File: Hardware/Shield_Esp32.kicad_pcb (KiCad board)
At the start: 2 copper layers, 93 x 70.5 mm, 43 parts, among them J1 Conn_01x02_Male, J10 Conn_01x02_Male, J11 Conn_01x02_Male, J12 Conn_01x02_Male, J13 Conn_01x02_Male, J14 Conn_01x02_Male, J15 Conn_01x02_Male, J16 Conn_01x02_Male, J17 Conn_01x02_Male, J18 Conn_01x02_Male, J19 Conn_01x02_Male, J2 Conn_01x02_Male, J20 Conn_01x02_Male, J21 Conn_01x02_Male, J22 Conn_01x02_Male, J23 Conn_01x02_Male, J3 Conn_02x13_Odd_Even, J4 Conn_01x15, J5 Conn_01x15, J6 Conn_01x02_Male, J7 Conn_01x02_Male, J8 Conn_01x03_Male, J9 Conn_01x02_Male

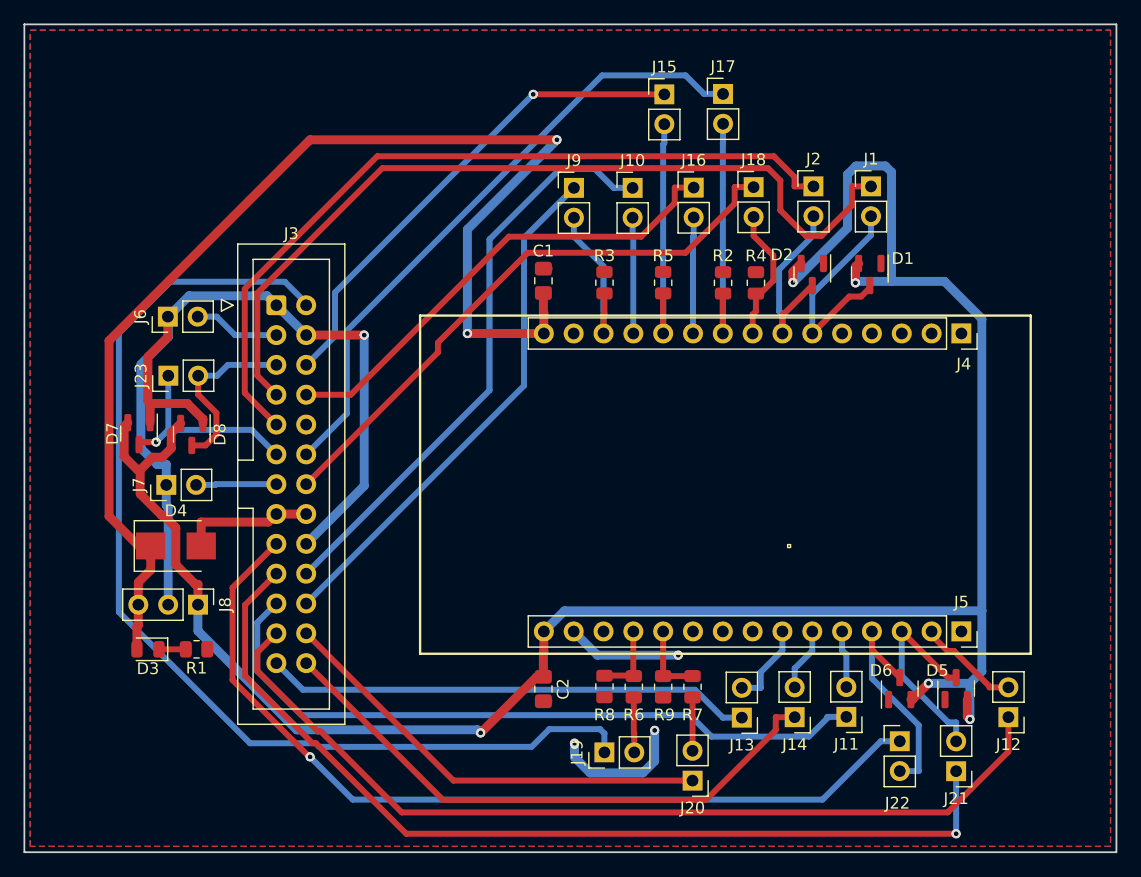
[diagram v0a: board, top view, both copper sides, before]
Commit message: pcb update
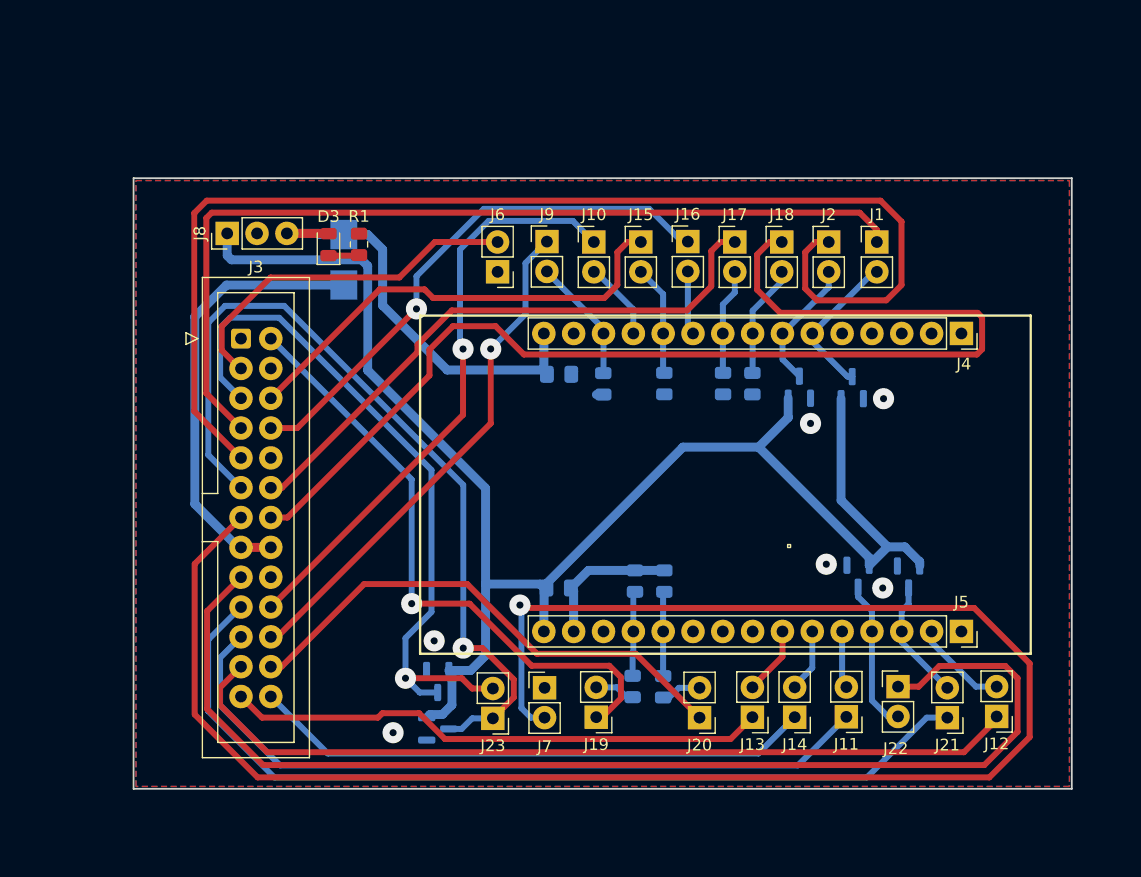
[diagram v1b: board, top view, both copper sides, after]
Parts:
- C1, C2, D1, D2, D4, D5, D6, D7, D8, R2, R3, R4, R5, R6, R7, R8, R9: moved to B.Cu
- moved J23 40.2 mm to (151.9, 120.1), turned to 180 degrees
- moved D3 37.7 mm to (137.9, 79.8), turned to 90 degrees
- moved R1 37.2 mm to (140.5, 79.7), turned to 90 degrees
- moved J7 36.6 mm to (156.3, 117.5), turned to 0 degrees
- moved D7 35.8 mm to (147.2, 121.0), turned to 0 degrees
- moved J8 31.7 mm to (129.3, 78.8), turned to 90 degrees
- moved D8 29.7 mm to (147.2, 117.0)
- moved J6 28.3 mm to (152.3, 82.1), turned to 180 degrees
- moved D4 28.3 mm to (139.2, 81.0), turned to -90 degrees
- moved J15 12.7 mm to (164.5, 79.5)
- moved J17 12.6 mm to (172.5, 79.5)
- moved D5 10.3 mm to (187.3, 108.1), turned to -90 degrees
- moved D6 10.2 mm to (183.0, 108.0), turned to -90 degrees
- moved D1 9.75 mm to (182.5, 91.9), turned to 90 degrees
- moved D2 9.66 mm to (178.0, 91.9), turned to 90 degrees
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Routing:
- net AMP2: track 6.86 -> 156.0 mm, vias 0 -> 1
- net GND: track 103.0 -> 13.3 mm, vias 4 -> 6
- net +5V: track 104.1 -> 36.6 mm, vias 2 -> 0
- net +3.3V: track 186.0 -> 132.3 mm, vias 5 -> 0
- net ADC2: track 17.7 -> 71.3 mm
- net L_TCRT: track 49.9 -> 98.2 mm
- net ADC3: track 15.2 -> 60.2 mm, vias 0 -> 1
- net ENC0: track 91.0 -> 52.5 mm, vias 0 -> 1
- net ADC1: track 67.3 -> 103.9 mm
- net +5VP: track 11.3 -> 37.8 mm
- net TXB: track 76.2 -> 100.5 mm, vias 1 -> 0
- net AMP1: track 7.35 -> 30.8 mm
- net D26: track 21.3 -> 9.03 mm
- net D14: track 21.3 -> 9.43 mm
- net TX0: track 17.9 -> 10.3 mm
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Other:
- board size 93 x 70.5 mm -> 79.9 x 52 mm
